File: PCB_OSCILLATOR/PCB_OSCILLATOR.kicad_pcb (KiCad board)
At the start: 2 copper layers, 96.8 x 43.9 mm, 96 parts, among them J1 Jumper, J10 Jumper, J11 Jumper, J12 Jumper, J13 Jumper, J14 Jumper, J15 Jumper, J16 Jumper, J2 Jumper, J3 Jumper, J4 Jumper, J5 Jumper, J6 Jumper, J7 Jumper, J8 Jumper, J9 Jumper, P1 CONN_01X04, P2 MCLK_EXTERNAL, P3 SPI_AD5270_1, P4 SPI_AD5270_2, P5 SPI_AD9833_1, P6 SPI_AD9833_2, P7 CONN_01X04, U1 AD5270, U10 ADR291, U2 AD8421, U3 AD9833, U4 AD5270, U5 AD8421, U6 AD9833, U7 ADG819, U8 ADP3303, U9 AD8651

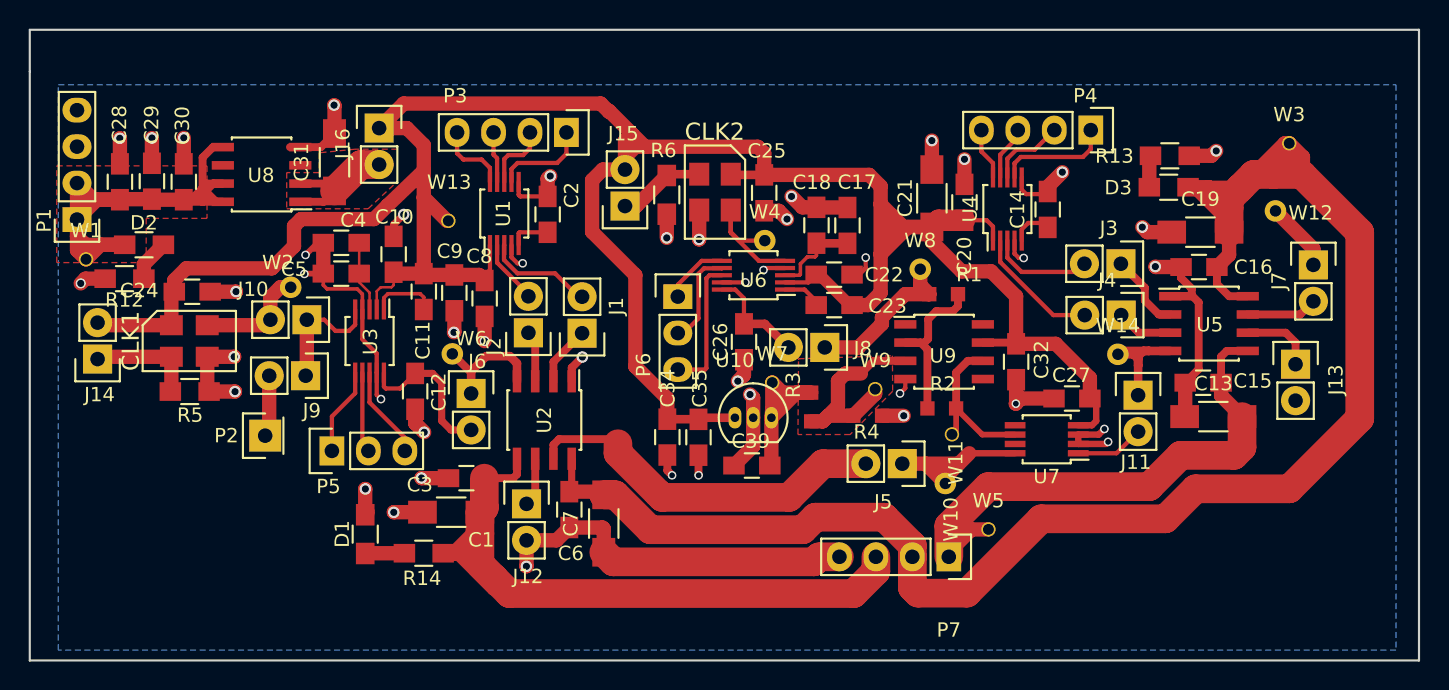
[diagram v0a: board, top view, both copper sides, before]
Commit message: 98% Completed
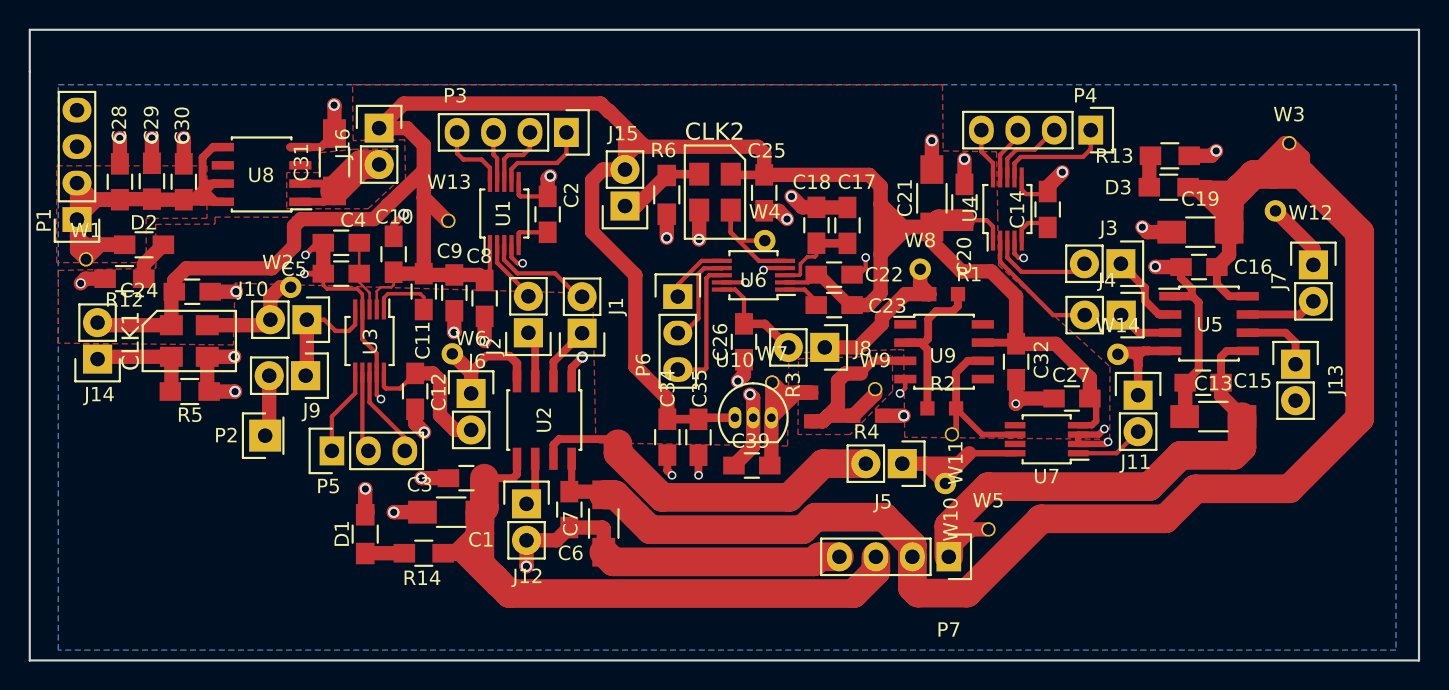
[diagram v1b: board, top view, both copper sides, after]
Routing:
- added copper zone on F.Cu, net /VDD
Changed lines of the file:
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@@
   )
   (setup
-    (last_trace_width 1)
+    (last_trace_width 0.45)
     (user_trace_width 0.3)
     (user_trace_width 0.35)
@@
     (user_trace_width 2)
     (trace_clearance 0.18)
-    (zone_clearance 0.3)
+    (zone_clearance 0.4)
     (zone_45_only no)
     (trace_min 0.1524)
@@
   (segment (start 85.15 79.95) (end 85.15 79.35) (width 0.1778) (layer F.Cu) (net 3))
   (segment (start 85.15 77.2) (end 85.15 79.35) (width 0.1778) (layer F.Cu) (net 3))
-  (segment (start 91.36 75.67) (end 91.28 75.67) (width 1) (layer F.Cu) (net 4) (status C00000))
-  (segment (start 91.28 75.67) (end 89.65 74.04) (width 1) (layer F.Cu) (net 4) (status 400000))
+  (segment (start 91.36 75.67) (end 91.28 75.67) (width 1) (layer F.Cu) (net 4))
+  (segment (start 91.28 75.67) (end 89.65 74.04) (width 1) (layer F.Cu) (net 4))
   (segment (start 91.78 79.44) (end 93.5 79.44) (width 1) (layer F.Cu) (net 4))
   (segment (start 93.5 79.44) (end 93.89 79.83) (width 1) (layer F.Cu) (net 4))
@@
   (segment (start 87.15 80.75) (end 89.4 80.75) (width 0.25) (layer F.Cu) (net 5))
   (segment (start 86.87232 81.02768) (end 87.15 80.75) (width 0.25) (layer F.Cu) (net 5))
-  (segment (start 92.95 90.24) (end 91.54 90.24) (width 0.5) (layer F.Cu) (net 6))
-  (segment (start 90.25 86.3) (end 89.05 86.3) (width 0.5) (layer F.Cu) (net 6))
-  (segment (start 90.9 86.95) (end 90.25 86.3) (width 0.5) (layer F.Cu) (net 6))
-  (segment (start 90.9 89.6) (end 90.9 86.95) (width 0.5) (layer F.Cu) (net 6))
-  (segment (start 91.54 90.24) (end 90.9 89.6) (width 0.5) (layer F.Cu) (net 6))
+  (segment (start 89.05 86.3) (end 90.28 86.3) (width 1) (layer F.Cu) (net 6))
+  (segment (start 91.81 90.24) (end 92.95 90.24) (width 1) (layer F.Cu) (net 6))
+  (segment (start 90.78 89.21) (end 91.81 90.24) (width 1) (layer F.Cu) (net 6))
+  (segment (start 90.78 86.8) (end 90.78 89.21) (width 1) (layer F.Cu) (net 6))
+  (segment (start 90.28 86.3) (end 90.78 86.8) (width 1) (layer F.Cu) (net 6))
   (segment (start 89.05 86.3) (end 89.2 86.3) (width 0.45) (layer F.Cu) (net 6))
   (segment (start 89.35 86.6) (end 89.05 86.3) (width 0.45) (layer F.Cu) (net 6))
@@
   (segment (start 94.76 78.59) (end 96.94 80.77) (width 0.3) (layer F.Cu) (net 31))
   (segment (start 96.94 80.77) (end 96.94 80.93) (width 0.3) (layer F.Cu) (net 31))
-  (segment (start 92.95 87.7) (end 92.95 86.25) (width 0.55) (layer F.Cu) (net 32))
-  (segment (start 92.95 86.25) (end 91.64 84.94) (width 0.55) (layer F.Cu) (net 32))
+  (segment (start 92.95 87.7) (end 92.95 86.25) (width 1) (layer F.Cu) (net 32))
+  (segment (start 92.95 86.25) (end 91.64 84.94) (width 1) (layer F.Cu) (net 32))
   (segment (start 96.145 86.85) (end 96.145 85.595) (width 0.6) (layer F.Cu) (net 32))
-  (segment (start 92.95 86.15) (end 92.95 87.7) (width 0.6) (layer F.Cu) (net 32))
-  (segment (start 94 85.1) (end 92.95 86.15) (width 0.6) (layer F.Cu) (net 32))
-  (segment (start 95.65 85.1) (end 94 85.1) (width 0.6) (layer F.Cu) (net 32))
   (segment (start 96.145 85.595) (end 95.65 85.1) (width 0.6) (layer F.Cu) (net 32))
+  (segment (start 95.65 85.1) (end 94 85.1) (width 0.6) (layer F.Cu) (net 32))
+  (segment (start 94 85.1) (end 92.95 86.15) (width 0.6) (layer F.Cu) (net 32))
+  (segment (start 92.95 86.15) (end 92.95 87.7) (width 0.6) (layer F.Cu) (net 32))
   (segment (start 130.31 77.05) (end 130.31 78.24) (width 0.3) (layer F.Cu) (net 33))
   (segment (start 131.3 79.23) (end 135.11 79.23) (width 0.3) (layer F.Cu) (net 33))
@@
       )
     )
+  )
+  (zone (net 4) (net_name /VDD) (layer F.Cu) (hatch edge 0.508)
+    (connect_pads (clearance 0.4))
+    (min_thickness 0.2)
+    (fill yes (arc_segments 16) (thermal_gap 0.508) (thermal_bridge_width 0.508) (smoothing fillet))
+    (polygon
+      (pts
+        (xy 125.79 66.19) (xy 125.84 70.8) (xy 129.56 70.86) (xy 129.64 75.29) (xy 129.68 78.74)
+        (xy 137.46 85.83) (xy 137.44 90.89) (xy 123.16 90.75) (xy 123.09 84.65) (xy 122.57 84.65)
+        (xy 115.09 84.88) (xy 115 91.36) (xy 101.64 91.14) (xy 101.42 80.73) (xy 76.5 80.01)
+        (xy 76.39 84.32) (xy 64.15 84.19) (xy 64.19 80.96) (xy 64.19 79.13) (xy 70.99 78.97)
+        (xy 70.97 75.92) (xy 75.1 75.9) (xy 75.11 75.84) (xy 75.11 75.71) (xy 75.1 75.41)
+        (xy 86.18 75.44) (xy 86.35 75.23) (xy 88.38 73.21) (xy 88.38 72.83) (xy 88.33 70.02)
+        (xy 84.73 70.08) (xy 84.69 66.18) (xy 125.79 66.19)
+      )
+    )
